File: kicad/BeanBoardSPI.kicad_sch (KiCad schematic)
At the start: 38 parts, among them J1 Power, J10 SPI6, J11 GPO, J12 GPO, J13 GPI, J14 GPI, J15 Power, J2 Address, J3 Data / Control, J4 SPI0 (RA8875), J5 SPI1, J6 SPI2, J7 SPI3, J8 SPI4, J9 SPI5, U1 74LS42, U10 74LS138, U2 74LS299, U3 74LS161, U4 74LS373, U5 74LS00, U6 74LS00, U7 74LS04, U8 74LS02, U9 74LS74

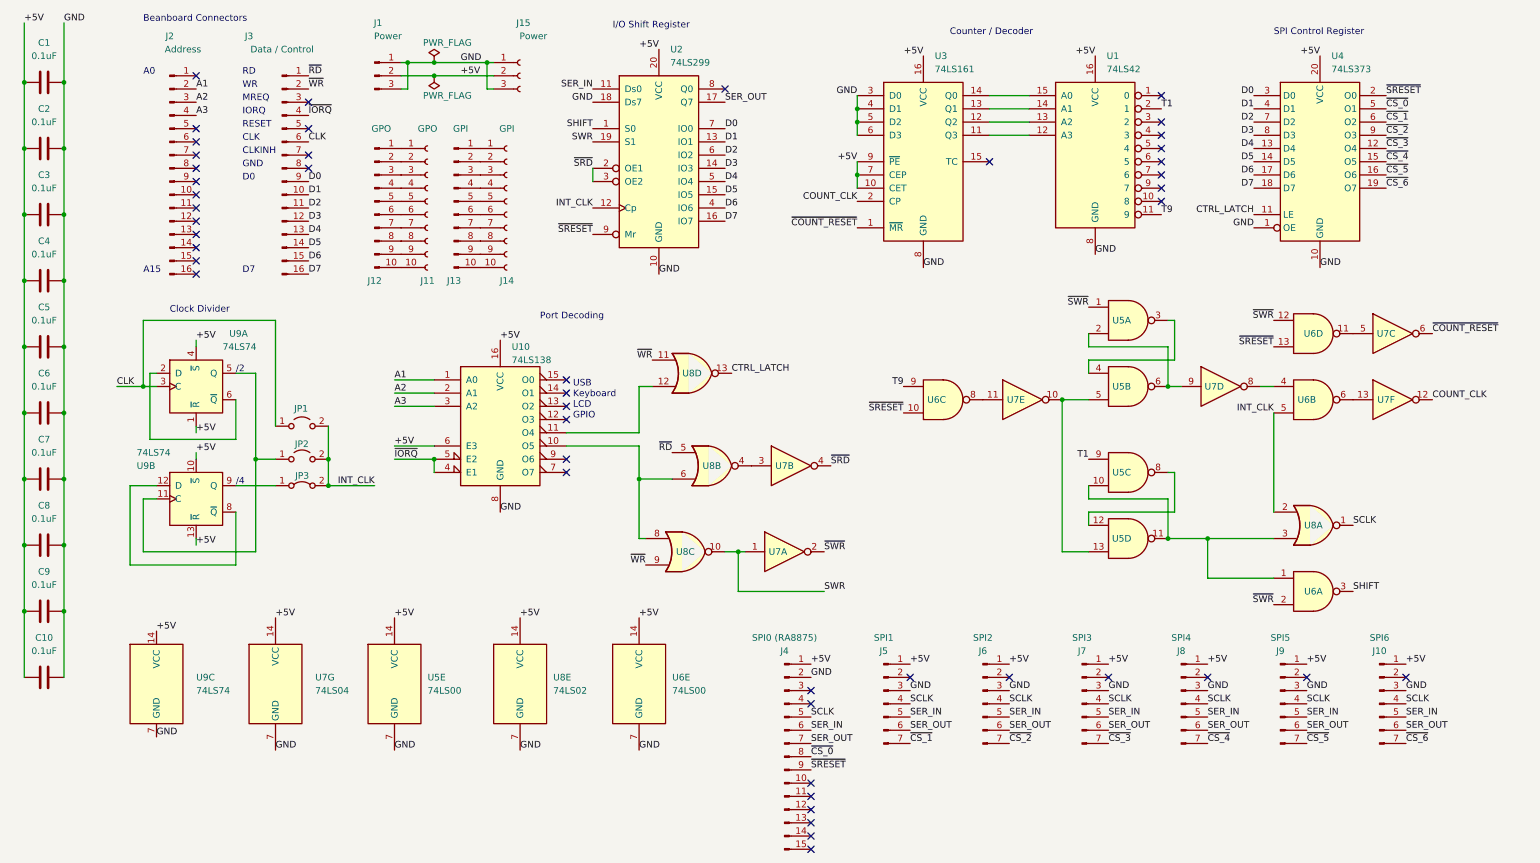
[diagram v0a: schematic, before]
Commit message: schematic
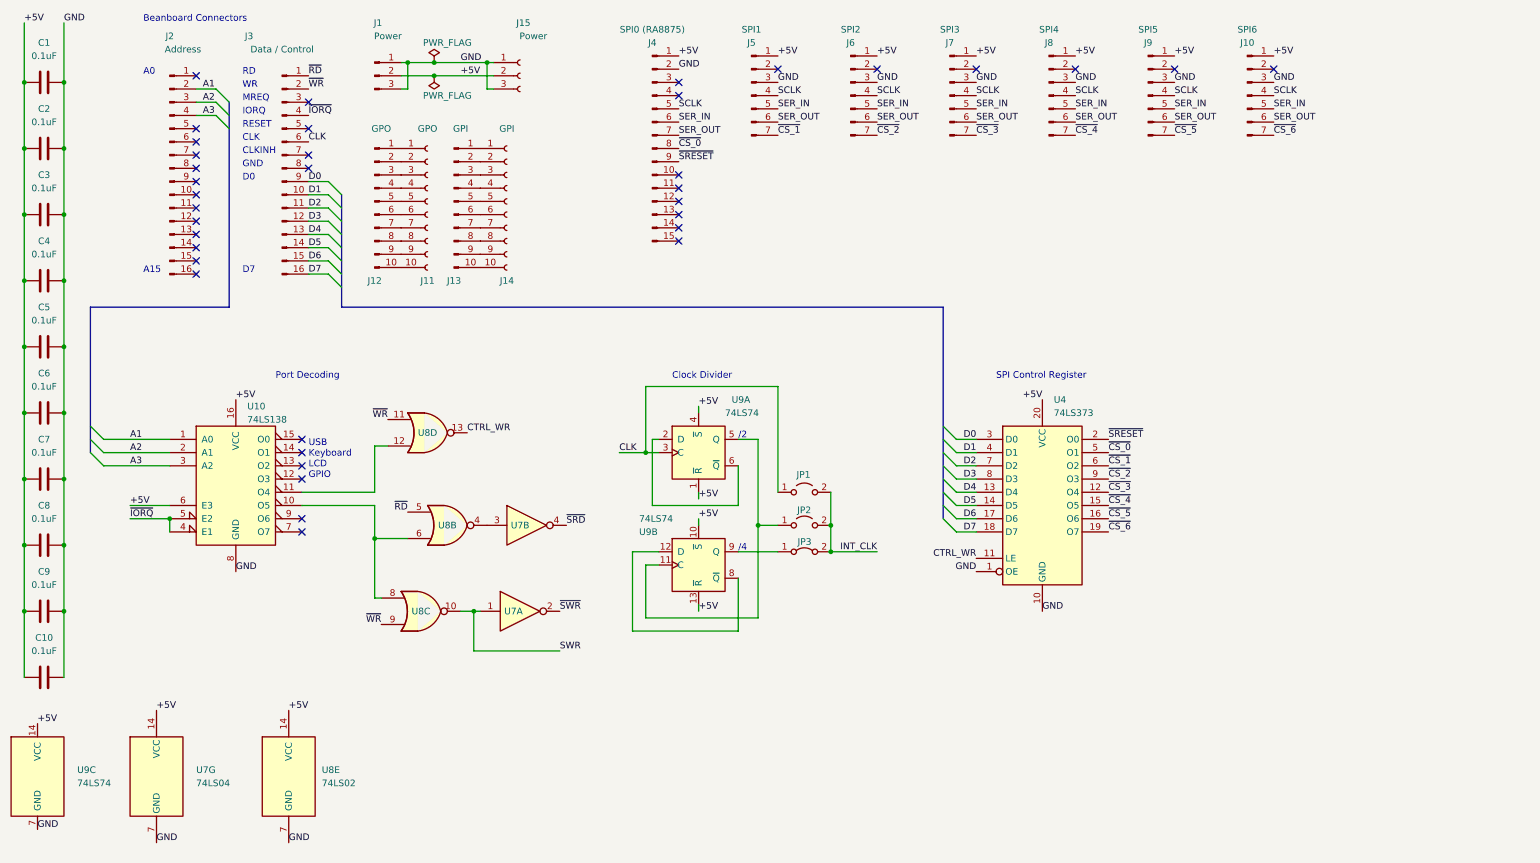
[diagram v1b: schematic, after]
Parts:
- removed U1: 74LS42, Package_DIP:DIP-16_W7.62mm_Socket, symbol 74xx:74LS42
- removed U2: 74LS299, Package_DIP:DIP-20_W7.62mm_Socket, symbol 74xx:74LS299
- removed U3: 74LS161, Package_DIP:DIP-16_W7.62mm_Socket, symbol 74xx:74LS161
- removed U5, U6: 74LS00, Package_DIP:DIP-14_W7.62mm_Socket, symbol 74xx:74LS00
- removed unit 4 of U7
- removed unit 3 of U7
- removed unit 6 of U7
- removed unit 5 of U7
- removed unit 1 of U8
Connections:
- net CTRL_LATCH renamed CTRL_WR
- no-connect marks 47 -> 37
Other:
- note removed: "Counter / Decoder"
- note removed: "I/O Shift Register"
- moved on the sheet: J10, J4, J5, J6, J7, J8, J9, JP1, JP2, JP3, U10, U4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
